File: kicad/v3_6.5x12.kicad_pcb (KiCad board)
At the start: 2 copper layers, 33.6 x 17.7 mm, 18 parts, among them J3 FDTI, SW1 SW_Push, U1 ATmega328P-A

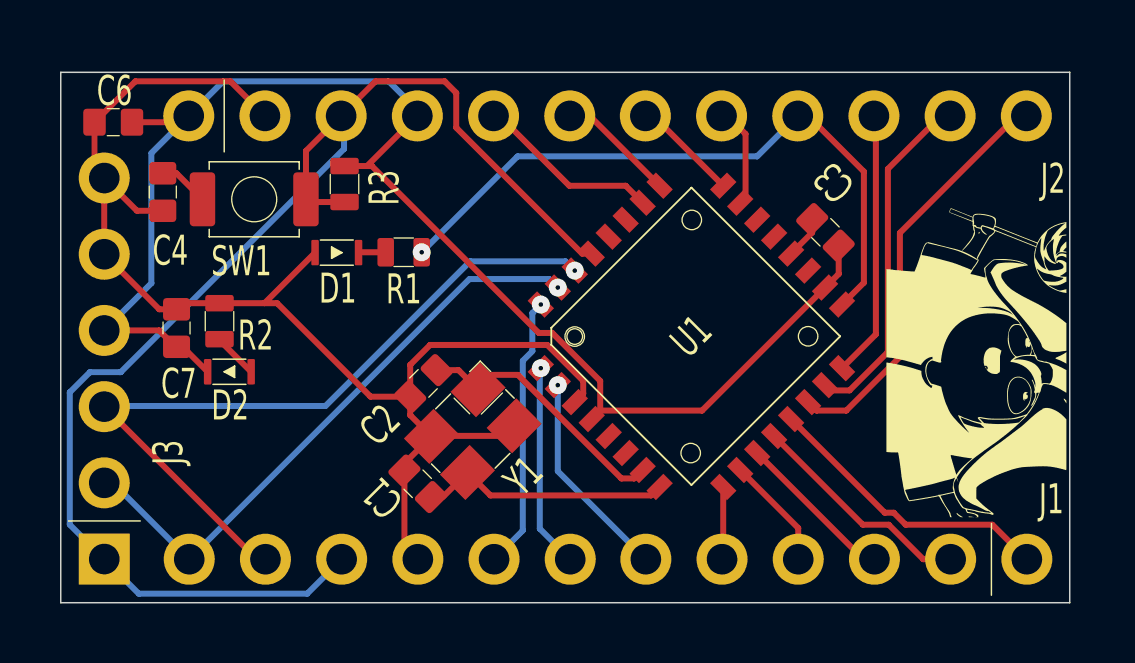
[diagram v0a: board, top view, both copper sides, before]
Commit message: Done ig
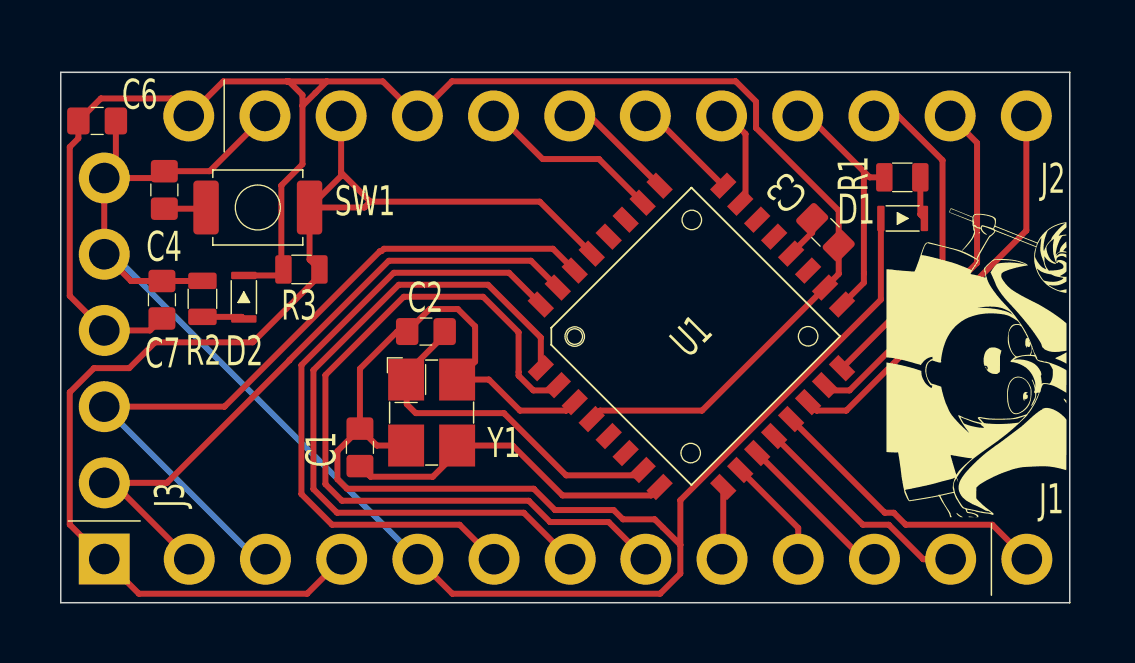
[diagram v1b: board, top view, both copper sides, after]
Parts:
- moved D1 18.9 mm to (77.5, 92.6)
- moved R1 16.8 mm to (77.5, 91.2), turned to 0 degrees
- moved R3 3.19 mm to (57.5, 94.3), turned to 0 degrees
- moved D2 2.53 mm to (55.6, 95.2), turned to 90 degrees
- moved C1 2.28 mm to (59.5, 100.2), turned to 90 degrees
- moved C2 1.73 mm to (61.6, 96.3), turned to 180 degrees
- moved Y1 1.51 mm to (61.8, 99.0), turned to -90 degrees
- moved C7 1.06 mm to (52.9, 95.3)
- moved R2 0.94 mm to (54.2, 95.2)
- moved C6 0.54 mm to (50.7, 89.3), turned to 0 degrees
- moved SW1 0.30 mm to (56.0, 92.2)
- moved C4 0.09 mm to (52.9, 91.6), turned to -90 degrees
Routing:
- net GND: track 45.2 -> 84.5 mm
- net D4: track 7.02 -> 26.7 mm, vias 1 -> 0
- net D3: track 6.47 -> 24.0 mm, vias 1 -> 0
- net SCK: track 22.4 -> 8.58 mm, vias 1 -> 0
- net D2: track 9.14 -> 21.3 mm, vias 1 -> 0
- net RAW: track 49.2 -> 61.0 mm
- net Net-(U1-XTAL2/PB7): track 8.00 -> 12.4 mm
- net Net-(U1-XTAL1/PB6): track 8.89 -> 12.4 mm
- net TXO: track 20.2 -> 22.7 mm, vias 1 -> 0
- net DTR: track 45.1 -> 42.6 mm
- net MISO: track 9.37 -> 11.2 mm
- net RXI: track 25.3 -> 26.0 mm, vias 1 -> 0
- net Net-(D1-Pad2): track 0.89 -> 1.43 mm

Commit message: a
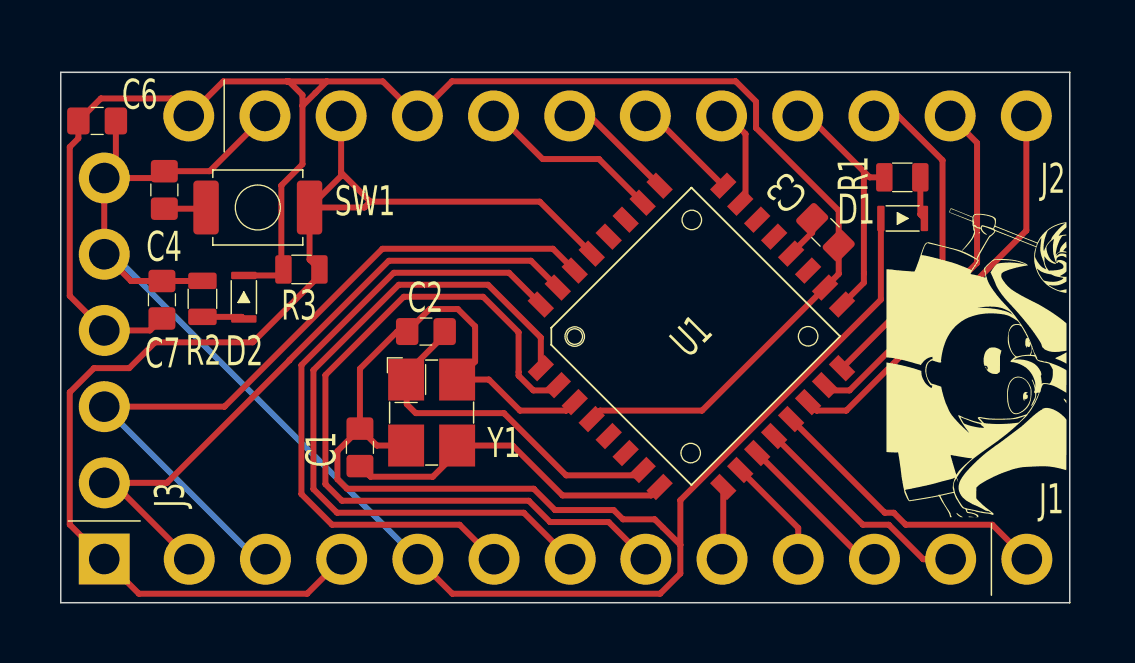
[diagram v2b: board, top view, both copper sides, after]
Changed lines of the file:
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@@
-	)
-	(segment
-		(start 54.936888 98.843112)
-		(end 60.12 93.66)
-		(width 0.2)
-		(layer "F.Cu")
-		(net "RXI")
-	)
-	(segment
-		(start 60.167258 93.66)
-		(end 60.247259 93.58)
-		(width 0.2)
-		(layer "F.Cu")
-		(net "RXI")
 	)
 	(segment
@@
 	)
 	(segment
-		(start 60.12 93.66)
-		(end 60.167258 93.66)
+		(start 50.927151 98.843112)
+		(end 54.936888 98.843112)
+		(width 0.2)
+		(layer "F.Cu")
+		(net "RXI")
+	)
+	(segment
+		(start 60.2 93.58)
+		(end 65.882944 93.58)
 		(width 0.2)
 		(layer "F.Cu")
@@
 	)
 	(segment
-		(start 60.247259 93.58)
-		(end 65.882944 93.58)
+		(start 54.936888 98.843112)
+		(end 60.2 93.58)
 		(width 0.2)
 		(layer "F.Cu")
-		(net "RXI")
-	)
-	(segment
-		(start 50.927151 98.843112)
-		(end 54.936888 98.843112)
-		(width 0.2)
-		(layer "F.Cu")
